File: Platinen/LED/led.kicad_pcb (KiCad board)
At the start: 2 copper layers, 3 parts, among them P1 CONN_2

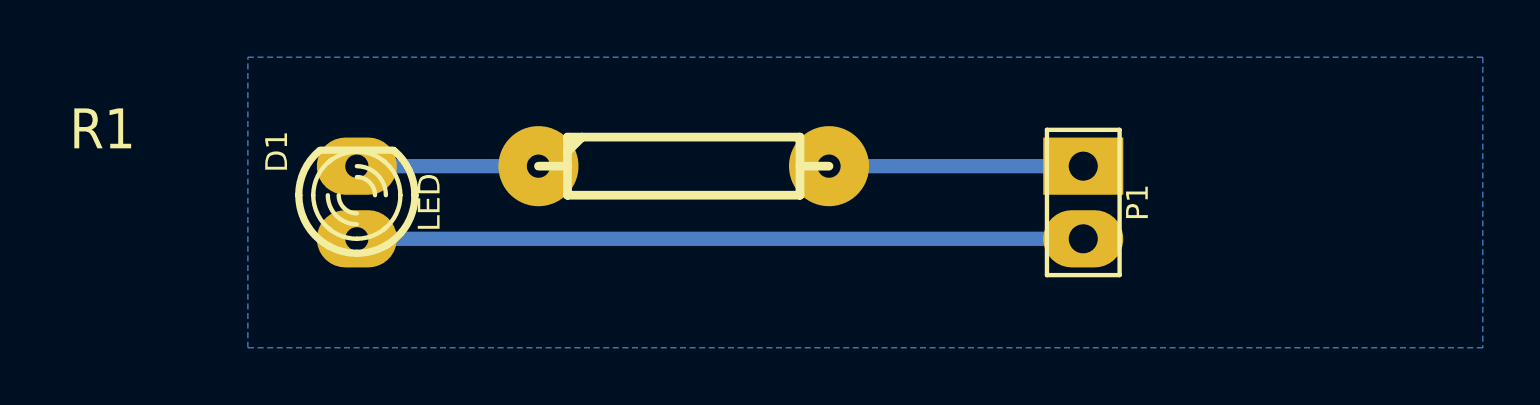
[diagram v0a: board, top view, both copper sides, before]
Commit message: Platinen aktuallisiert nach Ätzen der ersten Prototypplatine
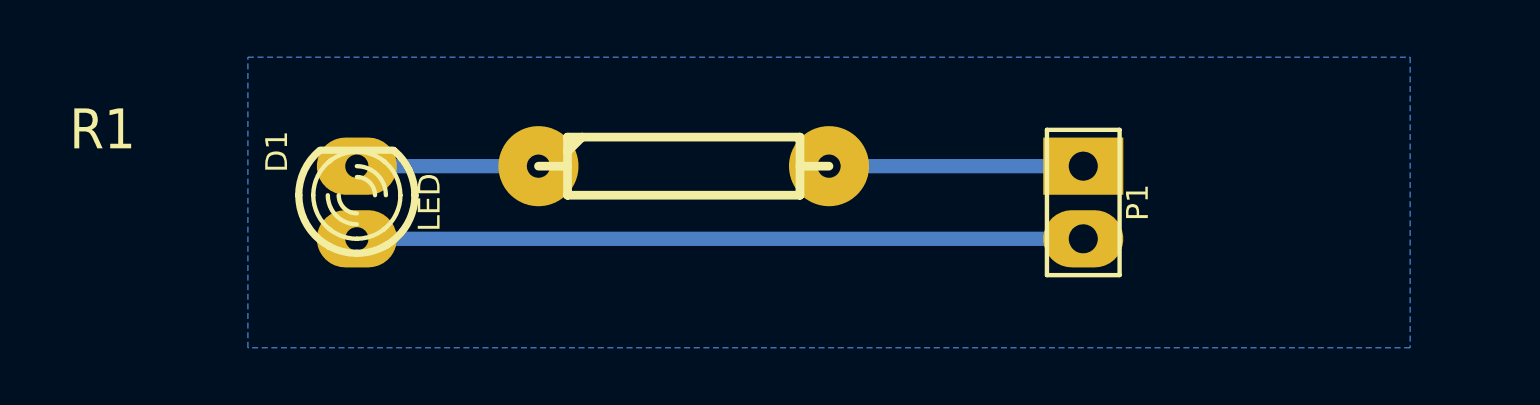
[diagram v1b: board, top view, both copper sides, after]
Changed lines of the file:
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@@
-(kicad_pcb (version 4) (host pcbnew 4.0.6-e0-6349~53~ubuntu14.04.1)
+(kicad_pcb (version 4) (host pcbnew 4.0.7-e2-6376~58~ubuntu16.04.1)
   (general
     (links 3)
     (no_connects 0)
-    (area 39.146238 46.9265 77.7748 53.670201)
+    (area 39.146238 39.91 88.900001 55.880001)
     (thickness 1.6)
-    (drawings 0)
+    (drawings 1)
     (tracks 3)
     (zones 0)
@@
     )
   )
+  (dimension 10.16 (width 0.25) (layer F.Adhes)
+    (gr_text "10,160 mm" (at 81.28 40.91) (layer F.Adhes)
+      (effects (font (size 1 1) (thickness 0.25)))
+    )
+    (feature1 (pts (xy 86.36 44.45) (xy 86.36 39.91)))
+    (feature2 (pts (xy 76.2 44.45) (xy 76.2 39.91)))
+    (crossbar (pts (xy 76.2 41.91) (xy 86.36 41.91)))
+    (arrow1a (pts (xy 86.36 41.91) (xy 85.233496 42.496421)))
+    (arrow1b (pts (xy 86.36 41.91) (xy 85.233496 41.323579)))
+    (arrow2a (pts (xy 76.2 41.91) (xy 77.326504 42.496421)))
+    (arrow2b (pts (xy 76.2 41.91) (xy 77.326504 41.323579)))
+  )
   (segment (start 49.53 52.07) (end 74.93 52.07) (width 0.5) (layer B.Cu) (net 1))
   (segment (start 55.88 49.53) (end 49.53 49.53) (width 0.5) (layer B.Cu) (net 2))
@@
     (polygon
       (pts
-        (xy 88.9 55.88) (xy 45.72 55.88) (xy 45.72 45.72) (xy 88.9 45.72)
+        (xy 86.36 55.88) (xy 45.72 55.88) (xy 45.72 45.72) (xy 86.36 45.72)
       )
     )

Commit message: Platinen überarbeitet
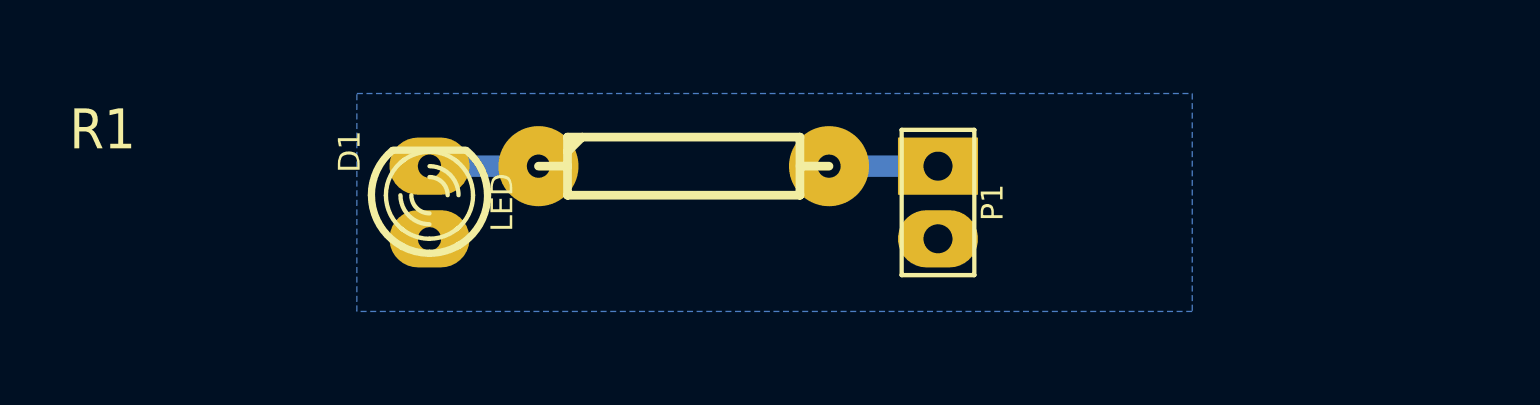
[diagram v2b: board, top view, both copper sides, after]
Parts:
- moved P1 5.08 mm to (69.8, 50.8)
- moved D1 2.54 mm to (52.1, 50.8)
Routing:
- net N-000001: track 25.4 -> 0.00 mm
- net N-000003: track 8.89 -> 3.81 mm
- net N-000002: track 6.35 -> 3.81 mm
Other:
- net class Default: trace_width 0.5 -> 0.75
- board text added: "GND"
- board text added: "PIN"
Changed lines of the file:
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@@
-(kicad_pcb (version 4) (host pcbnew 4.0.7-e2-6376~58~ubuntu16.04.1)
+(kicad_pcb (version 20171130) (host pcbnew 5.0.2-bee76a0~70~ubuntu16.04.1)
   (general
-    (links 3)
-    (no_connects 0)
-    (area 39.146238 39.91 88.900001 55.880001)
     (thickness 1.6)
-    (drawings 1)
-    (tracks 3)
+    (drawings 3)
+    (tracks 2)
     (zones 0)
     (modules 3)
@@
   )
   (setup
-    (last_trace_width 0.5)
+    (last_trace_width 0.75)
     (trace_clearance 0.254)
-    (zone_clearance 0.508)
+    (zone_clearance 0.8)
     (zone_45_only no)
     (trace_min 0.254)
@@
     (pad_drill 0.8128)
     (pad_to_mask_clearance 0)
-    (aux_axis_origin 0 0)
+    (solder_mask_min_width 0.25)
+    (aux_axis_origin 49.53 54.61)
+    (grid_origin 45.72 55.88)
     (visible_elements FFFFFFBF)
     (pcbplotparams
-      (layerselection 0x00030_80000001)
+      (layerselection 0x00008_fffffffe)
       (usegerberextensions true)
+      (usegerberattributes false)
+      (usegerberadvancedattributes false)
+      (creategerberjobfile false)
       (excludeedgelayer true)
       (linewidth 0.150000)
@@
       (viasonmask false)
       (mode 1)
-      (useauxorigin false)
+      (useauxorigin true)
       (hpglpennumber 1)
       (hpglpenspeed 20)
-      (hpglpendiameter 15)
-      (hpglpenoverlay 2)
+      (hpglpendiameter 15.000000)
       (psnegative false)
       (psa4output false)
-      (plotreference true)
-      (plotvalue true)
+      (plotreference false)
+      (plotvalue false)
       (plotinvisibletext false)
       (padsonsilk false)
@@
       (outputformat 1)
       (mirror false)
-      (drillshape 1)
+      (drillshape 0)
       (scaleselection 1)
       (outputdirectory ""))
@@
   (net_class Default "Dies ist die voreingestellte Netzklasse."
     (clearance 0.254)
-    (trace_width 0.5)
+    (trace_width 0.75)
     (via_dia 0.889)
     (via_drill 0.635)
@@
   )
   (module PIN_ARRAY_2X1 (layer F.Cu)
-    (at 74.93 50.8 270)
+    (at 69.85 50.8 270)
     (descr "Connecteurs 2 pins")
     (tags "CONN DEV")
@@
   )
   (module LED-3MM (layer F.Cu)
-    (at 49.53 50.8 90)
+    (at 52.07 50.8 90)
     (descr "LED 3mm - Lead pitch 100mil (2,54mm)")
     (tags "LED led 3mm 3MM 100mil 2,54mm")
@@
     )
   )
+  (gr_text PIN (at 72.39 49.53) (layer F.Paste)
+    (effects (font (size 1.8 1.8) (thickness 0.1)) (justify left))
+  )
+  (gr_text "GND\n" (at 72.39 52.07) (layer F.Paste)
+    (effects (font (size 1.8 1.8) (thickness 0.1)) (justify left))
+  )
   (dimension 10.16 (width 0.25) (layer F.Adhes)
     (gr_text "10,160 mm" (at 81.28 40.91) (layer F.Adhes)
@@
     (arrow2b (pts (xy 76.2 41.91) (xy 77.326504 41.323579)))
   )
-  (segment (start 49.53 52.07) (end 74.93 52.07) (width 0.5) (layer B.Cu) (net 1))
-  (segment (start 55.88 49.53) (end 49.53 49.53) (width 0.5) (layer B.Cu) (net 2))
-  (segment (start 74.93 49.53) (end 66.04 49.53) (width 0.5) (layer B.Cu) (net 3))
+  (segment (start 55.88 49.53) (end 52.07 49.53) (width 0.75) (layer B.Cu) (net 2))
+  (segment (start 69.85 49.53) (end 66.04 49.53) (width 0.75) (layer B.Cu) (net 3) (status 30))
   (zone (net 1) (net_name N-000001) (layer B.Cu) (hatch edge 0.508)
-    (connect_pads (clearance 0.508))
-    (min_thickness 0.254)
-    (fill yes (arc_segments 16) (thermal_gap 0.508) (thermal_bridge_width 0.508))
+    (connect_pads (clearance 0.8))
+    (min_thickness 0.7)
+    (fill yes (arc_segments 16) (thermal_gap 0.8) (thermal_bridge_width 0.8))
     (polygon
       (pts
-        (xy 86.36 55.88) (xy 45.72 55.88) (xy 45.72 45.72) (xy 86.36 45.72)
+        (xy 78.74 54.61) (xy 49.53 54.61) (xy 49.53 46.99) (xy 78.74 46.99)
       )
     )
